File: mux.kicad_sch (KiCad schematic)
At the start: 22 parts, among them M1 SN74LV4051ADYYR, M10 SN74LV4051ADYYR, M11 SN74LV4051ADYYR, M2 SN74LV4051ADYYR, M3 SN74LV4051ADYYR, M4 SN74LV4051ADYYR, M5 SN74LV4051ADYYR, M6 SN74LV4051ADYYR, M7 SN74LV4051ADYYR, M8 SN74LV4051ADYYR, M9 SN74LV4051ADYYR

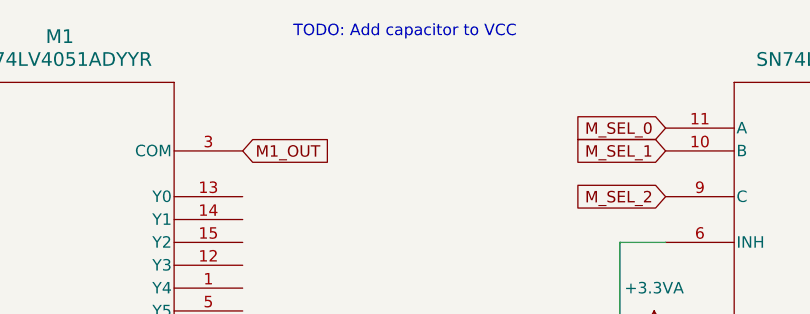
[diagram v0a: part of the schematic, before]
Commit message: final switch layout
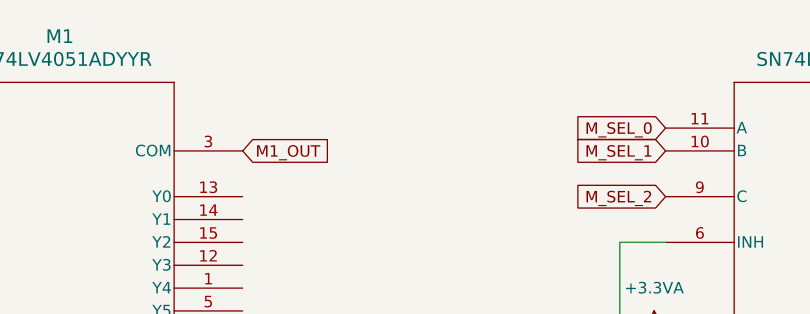
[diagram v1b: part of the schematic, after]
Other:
- note removed: "TODO: Add capacitor to VCC"
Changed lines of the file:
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@@
 		(title "Multiplexers")
-	)
-	(text "TODO: Add capacitor to VCC"
-		(exclude_from_sim no)
-		(at 87.884 18.542 0)
-		(effects
-			(font
-				(size 1.27 1.27)
-			)
-		)
 	)
 	(junction
